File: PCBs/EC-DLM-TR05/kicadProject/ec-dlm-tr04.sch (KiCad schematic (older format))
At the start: 20 parts, among them J1 input, J2 LED Connector, J3 RJ45, U1 TL074

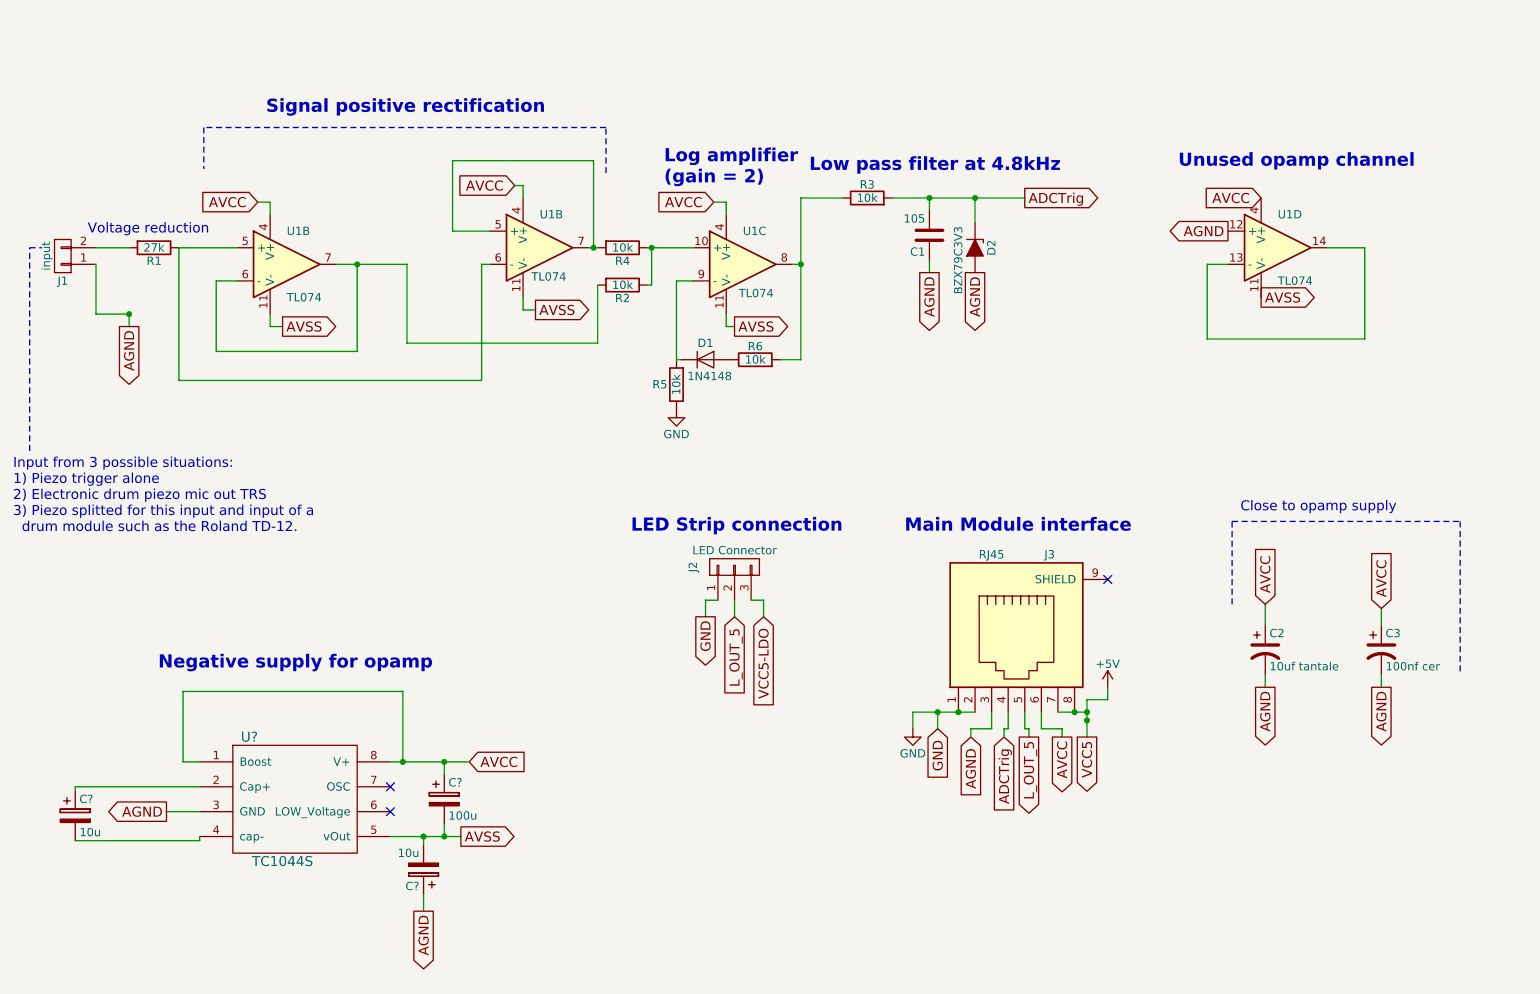
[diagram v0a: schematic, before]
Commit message: Revision board rev9
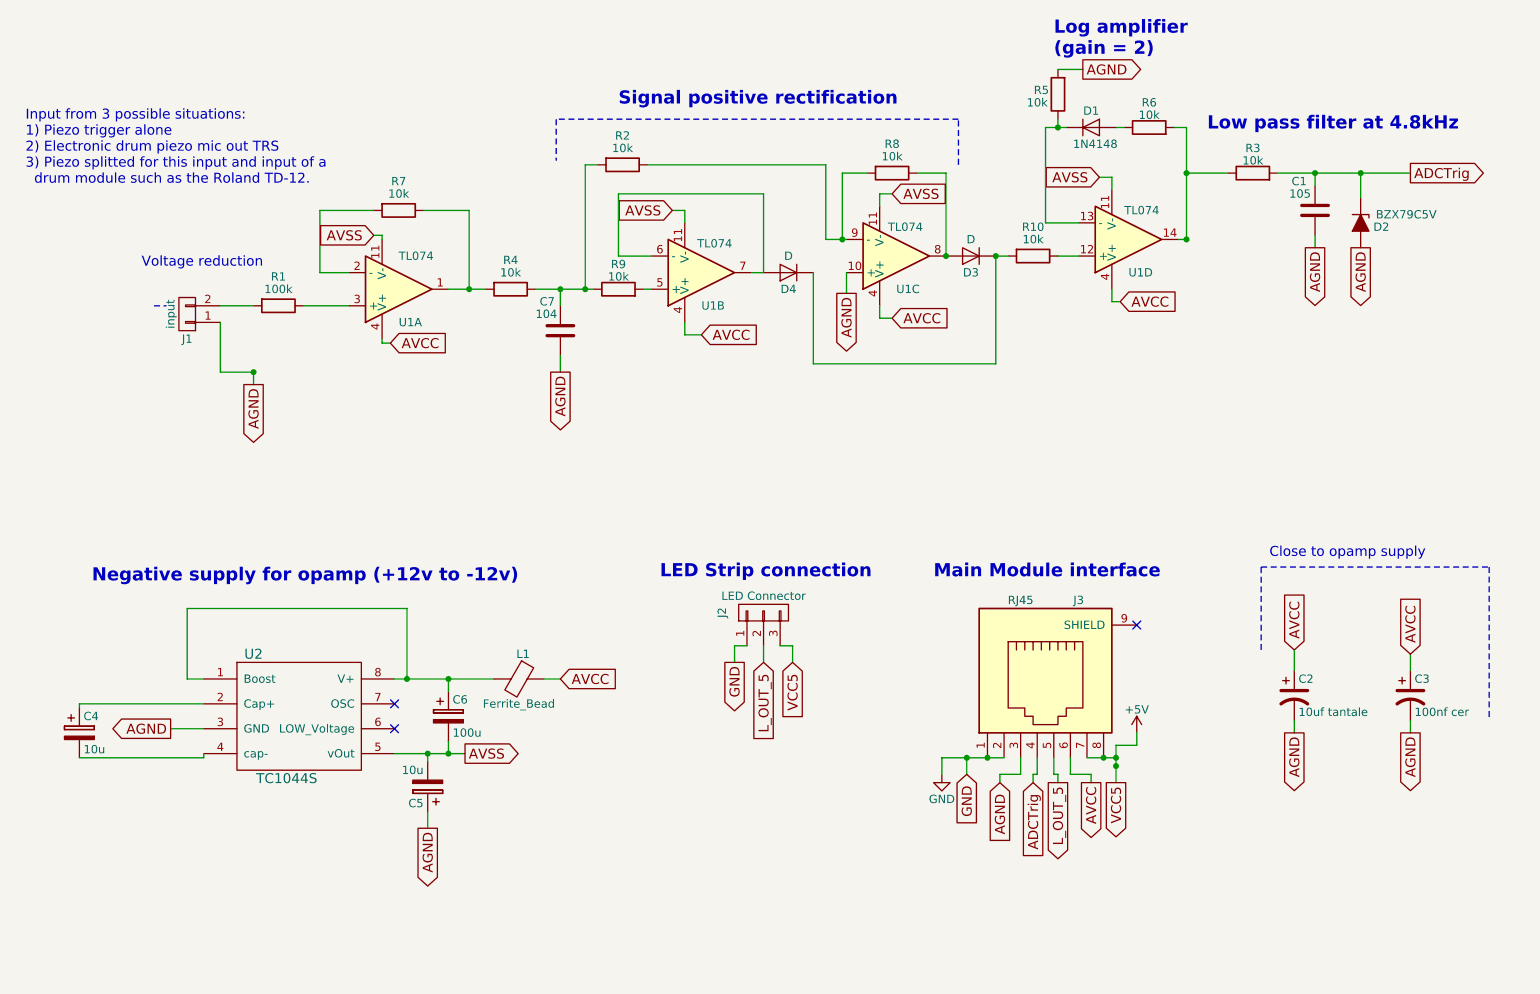
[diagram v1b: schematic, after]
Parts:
- added C7: 104, Capacitors_THT:CP_Radial_D6.3mm_P2.50mm, symbol C
- added D3, D4: D, Diodes_THT:D_A-405_P2.54mm_Vertical_AnodeUp, symbol D
- added L1: Ferrite_Bead, Inductors_THT:L_Axial_L6.6mm_D2.7mm_P2.54mm_Vertical_Vishay_IM-2, symbol Ferrite_Bead
- added R10, R7, R8, R9: 10k, Resistors_THT:R_Axial_DIN0204_L3.6mm_D1.6mm_P1.90mm_Vertical, symbol R
- C4, C5, C6: renamed from C?; footprint (none) -> Capacitors_THT:CP_Radial_D6.3mm_P2.50mm
- D2: value BZX79C3V3 -> BZX79C5V; footprint Diodes_THT:D_DO-35_SOD27_P7.62mm_Horizontal -> Diodes_THT:D_DO-35_SOD27_P2.54mm_Vertical_AnodeUp
- R1: value 27k -> 100k; footprint Resistors_THT:R_Axial_DIN0207_L6.3mm_D2.5mm_P7.62mm_Horizontal -> Resistors_THT:R_Axial_DIN0204_L3.6mm_D1.6mm_P1.90mm_Vertical
- R2, R3, R4, R5, R6: footprint Resistors_THT:R_Axial_DIN0207_L6.3mm_D2.5mm_P7.62mm_Horizontal -> Resistors_THT:R_Axial_DIN0204_L3.6mm_D1.6mm_P1.90mm_Vertical
- U2: renamed from U?; footprint (none) -> Housings_SOIC:SOIC-8_3.9x4.9mm_Pitch1.27mm
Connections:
- net VCC5-LDO is gone; now on net +5V: J2.3 (P3)
- net AGND: now also R5.2, U1.10 (+), C7.2; no longer U1.12 (+)
- net AVCC: now also L1.1; no longer C6.1, U2.1 (Boost), U2.8 (V+)
- net GND: no longer R5.1
- net at U1.6 (-), U1.7: now also D4.2 (A); no longer R2.2
- net at R3.1, R6.2: now also U1.14; no longer U1.8
- new net: R9.2, U1.5 (+)
- new net: D3.2 (A), R8.1, U1.8
- new net: R2.1, R8.2, U1.9 (-)
- new net: R10.1, U1.12 (+)
- new net: D1.1 (K), R5.1, U1.13 (-)
- new net: R4.2, R7.1, U1.1
- new net: R7.2, U1.2 (-)
- new net: R1.1, U1.3 (+)
- new net: C7.1, R2.2, R4.1, R9.1
- new net: C6.1, L1.2, U2.1 (Boost), U2.8 (V+)
- new net: D3.1 (K), D4.1 (K), R10.2
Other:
- note added: "Negative supply for opamp (+12v to -12v)"
- note removed: "Negative supply for opamp"
- note removed: "Unused opamp channel"
- moved on the sheet: C1, C2, C3, C4, C5, C6, D1, D2, J1, J2, J3, R1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
